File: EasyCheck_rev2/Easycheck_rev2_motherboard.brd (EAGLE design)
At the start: 80 x 107 mm, 61 parts, among them J1 DC-044-20A, J2 CORTEX_DEBUG_PTH, Q1 DMG3415U, Q2 SI7465DP, T1 DS18B20, T2 MMBT2222A, U1 LM5085, U2 AP2114H-3.3V- 1A, U3 ATSAMD21G18A-AU, X1 JST-XH-02, X3 32.768

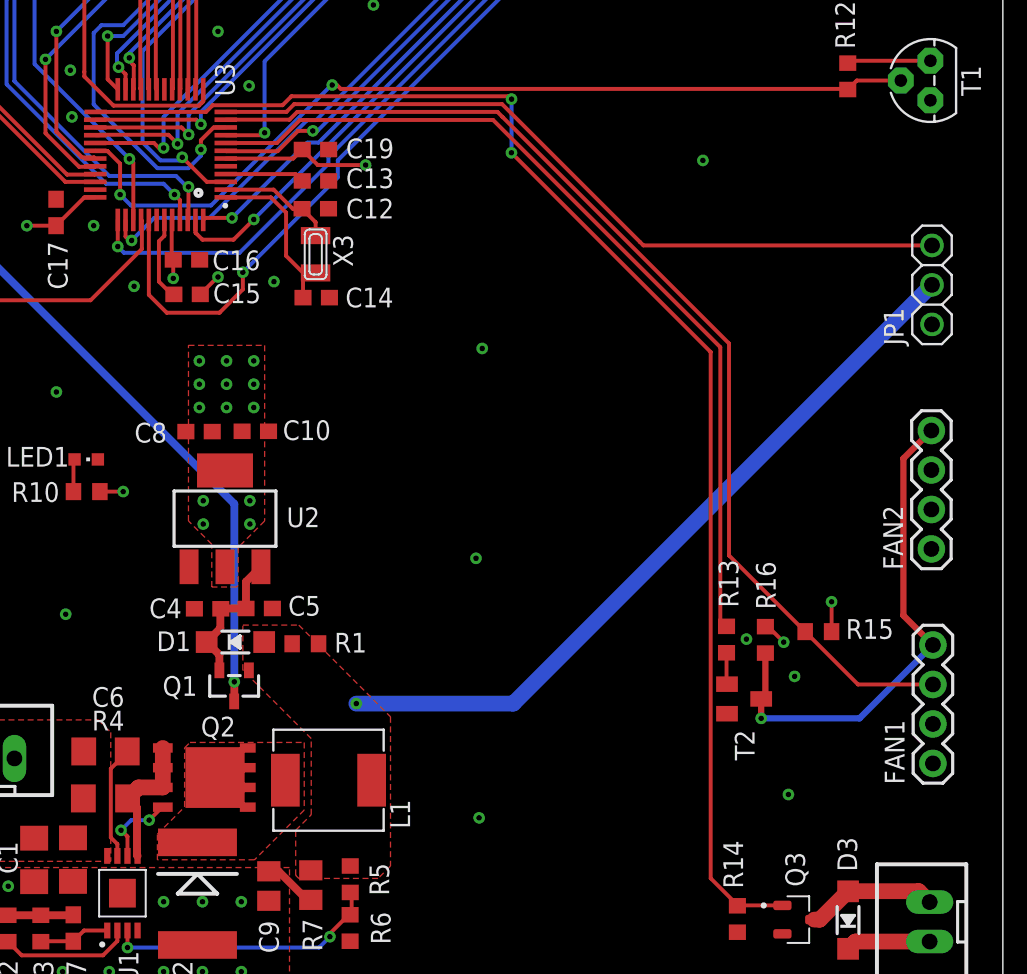
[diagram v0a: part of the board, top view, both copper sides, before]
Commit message: Corrected hardware files
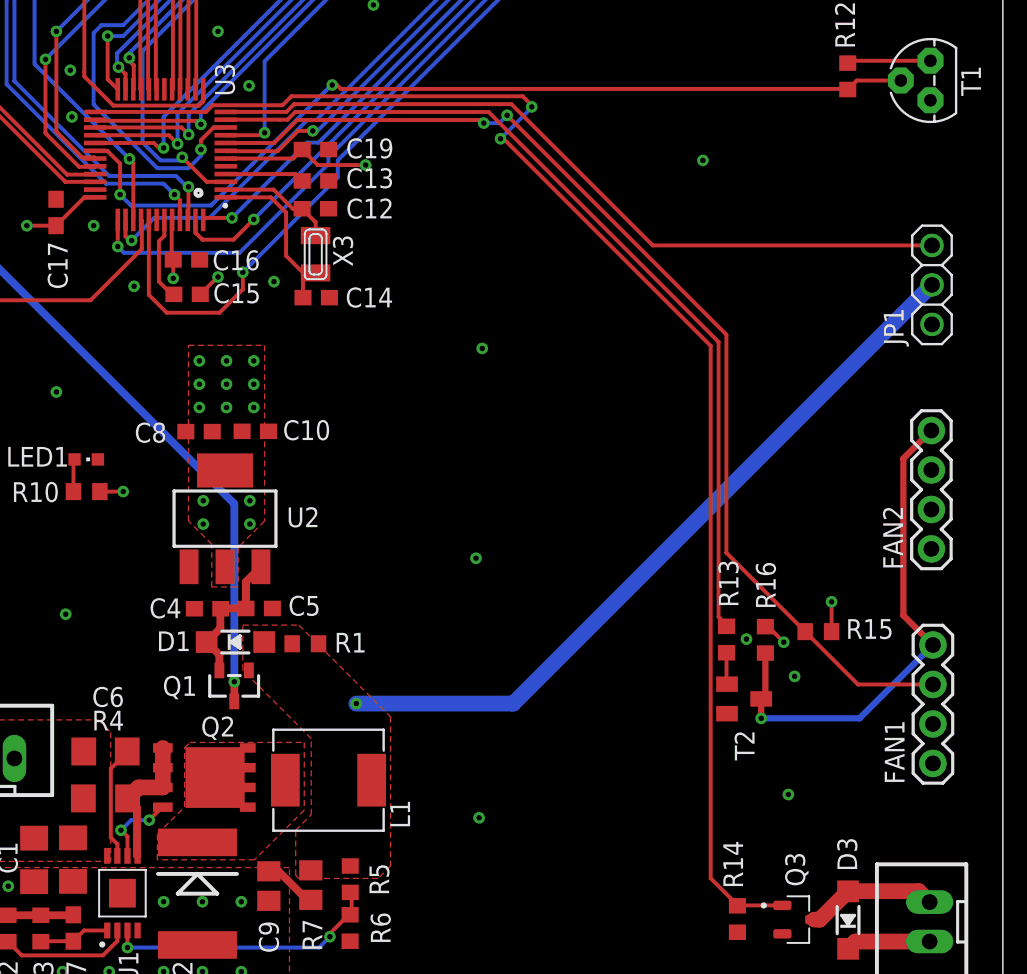
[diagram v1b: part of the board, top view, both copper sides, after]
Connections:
- net /SS: now also JP2.7, U3.27; no longer JP2.9, U3.28
- net FAN0: now also U3.11; no longer U3.8
- net FAN0_SPEED: now also U3.8; no longer U3.11
- net MOSI: now also JP2.9, U3.28; no longer JP2.5, U3.26
- net SCK: now also JP2.5, U3.26; no longer JP2.7, U3.27
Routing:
- net MOSI: track 61.6 -> 64.1 mm
- net HEATER0: track 88.1 -> 90.4 mm
- net /SS: track 63.4 -> 61.6 mm
- net FAN0_SPEED: track 69.0 -> 70.4 mm, vias 0 -> 2
